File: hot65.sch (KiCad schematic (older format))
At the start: 158 parts, among them P1 USB_C_Plug_USB2.0, SW1 SW_Push, SW10 SW_Push, SW11 SW_Push, SW12 SW_Push, SW13 SW_Push, SW14 SW_Push, SW15 SW_Push, SW16 SW_Push, SW17 SW_Push, SW18 SW_Push, SW19 SW_Push, SW2 SW_Push, SW20 SW_Push, SW21 SW_Push, SW22 SW_Push, SW23 SW_Push, SW24 SW_Push, SW25 SW_Push, SW26 SW_Push, SW27 SW_Push, SW28 SW_Push, SW29 SW_Push, SW3 SW_Push, SW30 SW_Push, SW31 SW_Push, SW32 SW_Push, SW33 SW_Push, SW34 SW_Push, SW35 SW_Push, SW36 SW_Push, SW37 SW_Push, SW38 SW_Push, SW39 SW_Push, SW4 SW_Push, SW40 SW_Push, SW41 SW_Push, SW42 SW_Push, SW43 SW_Push, SW44 SW_Push, SW45 SW_Push, SW46 SW_Push, SW47 SW_Push, SW48 SW_Push, SW49 SW_Push, SW5 SW_Push, SW50 SW_Push, SW51 SW_Push, SW52 SW_Push, SW53 SW_Push, SW54 SW_Push, SW55 SW_Push, SW56 SW_Push, SW57 SW_Push, SW58 SW_Push, SW59 SW_Push, SW6 SW_Push, SW60 SW_Push, SW61 SW_Push, SW62 SW_Push, SW63 SW_Push, SW64 SW_Push, SW65 SW_Push, SW66 SW_Push, SW67 SW_Push, SW68 SW_Push, SW7 SW_Push, SW8 SW_Push, SW9 SW_Push, U1 ATmega32U4-AU, Y1 Crystal_Small

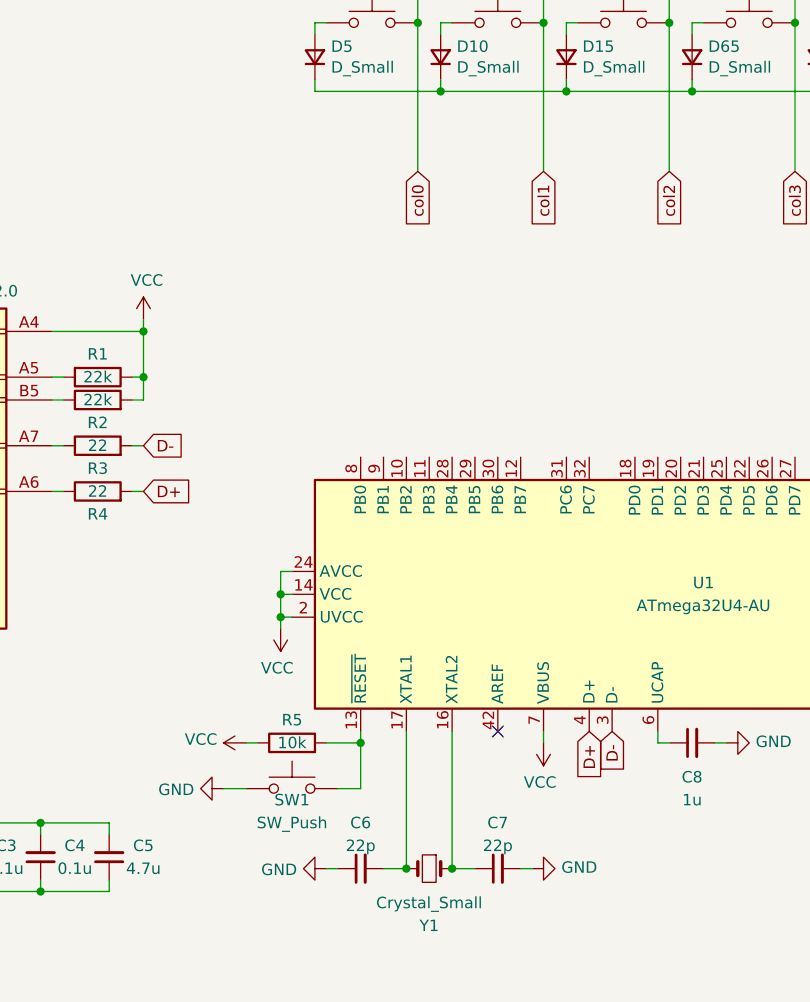
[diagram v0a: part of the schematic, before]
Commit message: v.0.7
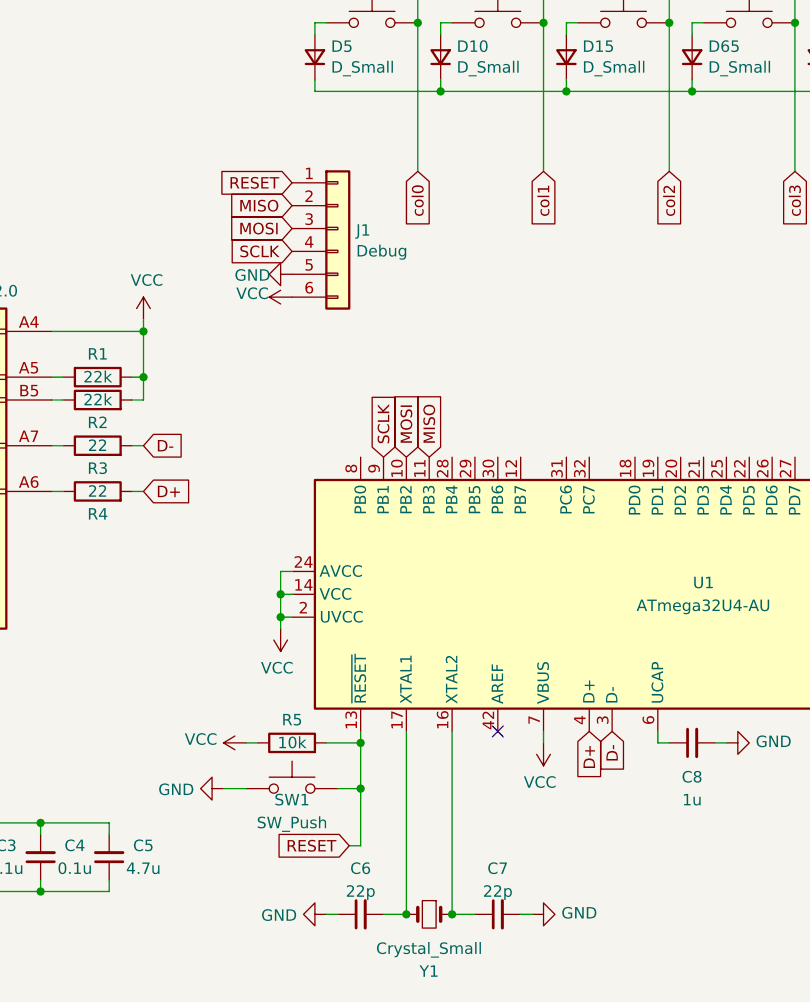
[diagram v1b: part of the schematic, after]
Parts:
- added J1: Debug, Connector_PinHeader_1.00mm:PinHeader_1x06_P1.00mm_Vertical, symbol Connector_Generic:Conn_01x06
- D1, D10, D11, D12, D13, D14, D15, D16, D17, D18, D19, D2, D20, D21, D22, D23, D24, D25, D26, D27, D28, D29, D3, D30, D31, D32, D33, D34, D35, D36, D37, D38, D39, D4, D40, D41, D42, D43, D44, D45, D46, D47, D48, D49, D5, D50, D51, D52, D53, D54, D55, D56, D57, D58, D59, D6, D60, D61, D62, D63, D64, D65, D66, D67, D7, D8, D9: footprint Diode_THT:D_A-405_P5.08mm_Vertical_AnodeUp -> Diode_THT:D_T-1_P5.08mm_Horizontal
- SW10, SW12, SW13, SW14, SW15, SW17, SW18, SW19, SW2, SW20, SW21, SW22, SW23, SW24, SW25, SW26, SW27, SW28, SW30, SW31, SW32, SW33, SW34, SW35, SW36, SW37, SW38, SW39, SW40, SW41, SW42, SW43, SW44, SW45, SW46, SW47, SW48, SW49, SW50, SW51, SW52, SW53, SW54, SW55, SW56, SW57, SW58, SW59, SW60, SW64, SW65, SW7, SW8, SW9: footprint keyswitches:Socket MX Alps -> MXSocketAlps:MXSocketAlps
- SW11, SW16, SW6: footprint keyswitches:Socket MX Alps -> MXSocketAlps:MXSocketAlps_1.25u
- SW29: footprint keyboardstuff:MXSocketAlps_6.25u -> MXSocketAlps:MXSocketAlps_6.25u
- SW3, SW62: footprint keyswitches:Socket MX Alps -> MXSocketAlps:MXSocketAlps_1.5u
- SW4: footprint keyswitches:Socket MX Alps -> MXSocketAlps:MXSocketAlps _1.75u
- SW5, SW61, SW66: footprint keyboardstuff:MXSocketAlps_2u -> MXSocketAlps:MXSocketAlps_2u
- SW63: footprint keyboardstuff:MXSocketAlps_2.25u -> MXSocketAlps:MXSocketAlps_2.25u
- SW67: footprint keyboardstuff:MXSocketAlps -> MXSocketAlps:MXSocketAlps_1.25u
- SW68: footprint keyboardstuff:MXSocketAlps_6.25u -> MXSocketAlps:MXSocketAlps_3u
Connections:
- net GND: now also J1.5 (Pin_5)
- net VCC: now also J1.6 (Pin_6)
- net MOSI: now reaches U1.10 (PB2)
- net MOSI: now also J1.3 (Pin_3)
- net MISO: now reaches U1.11 (PB3)
- net MISO: now also J1.2 (Pin_2)
- net RESET: now reaches R5.2, SW1.2, U1.13 (~RESET)
- net RESET: now also J1.1 (Pin_1)
- net SCLK: now reaches U1.9 (PB1)
- net SCLK: now also J1.4 (Pin_4)
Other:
- moved on the sheet: C6, C7, Y1

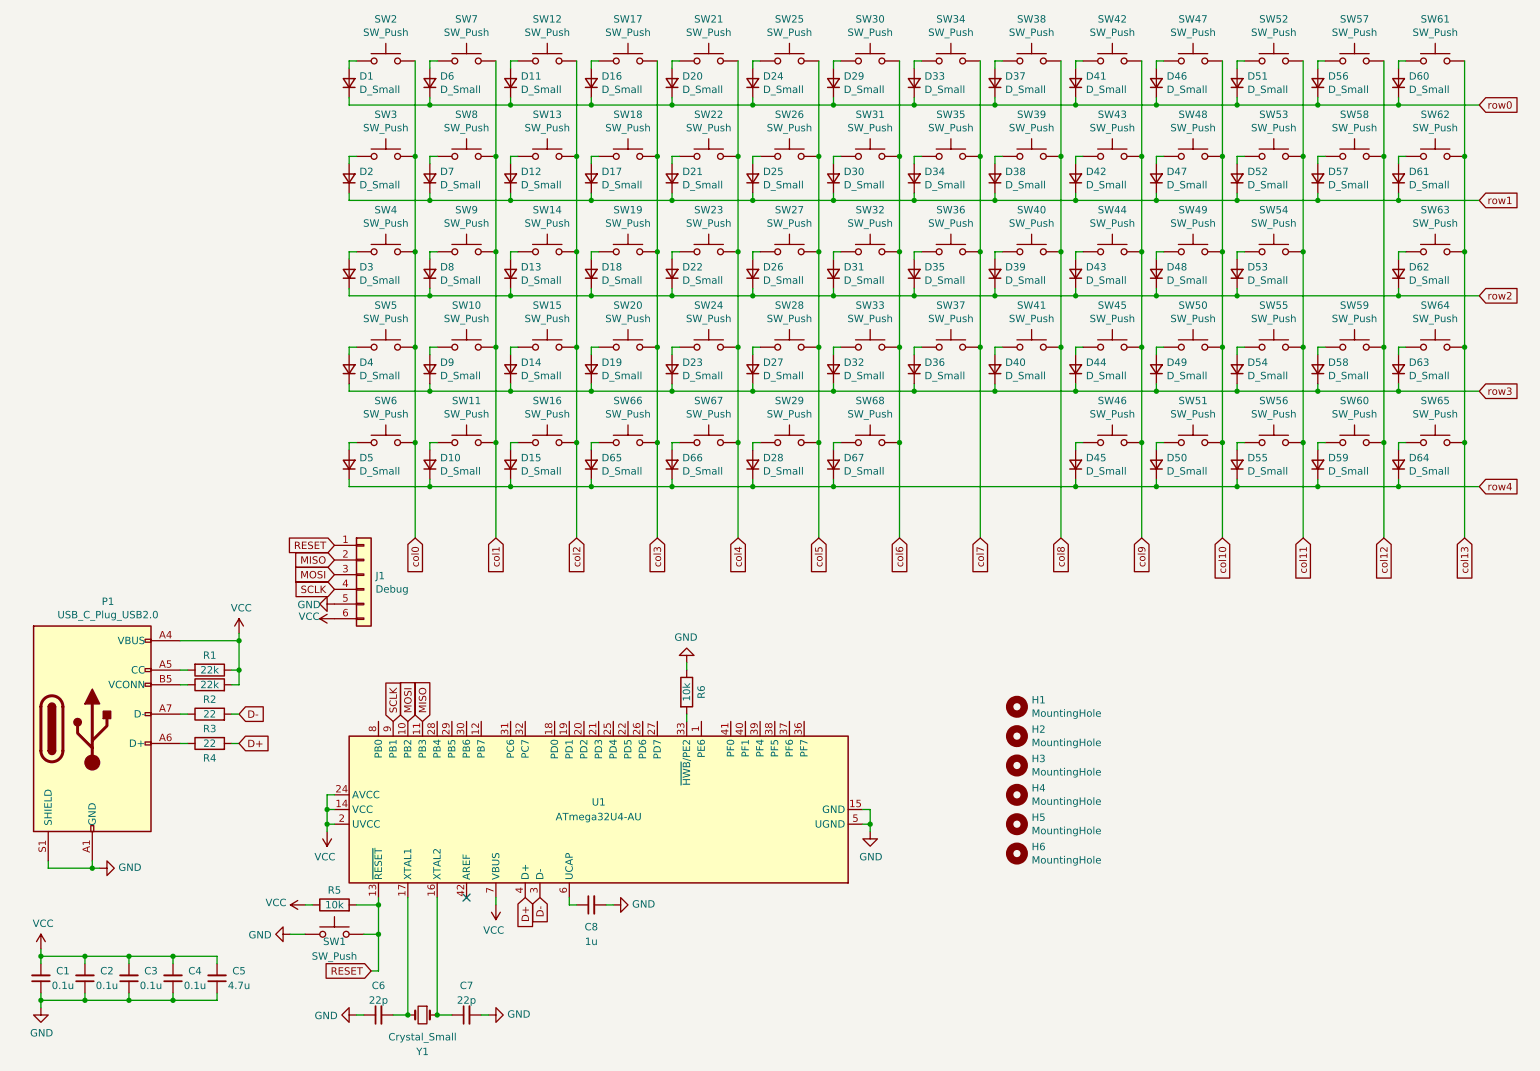
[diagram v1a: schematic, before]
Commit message: v.1.0
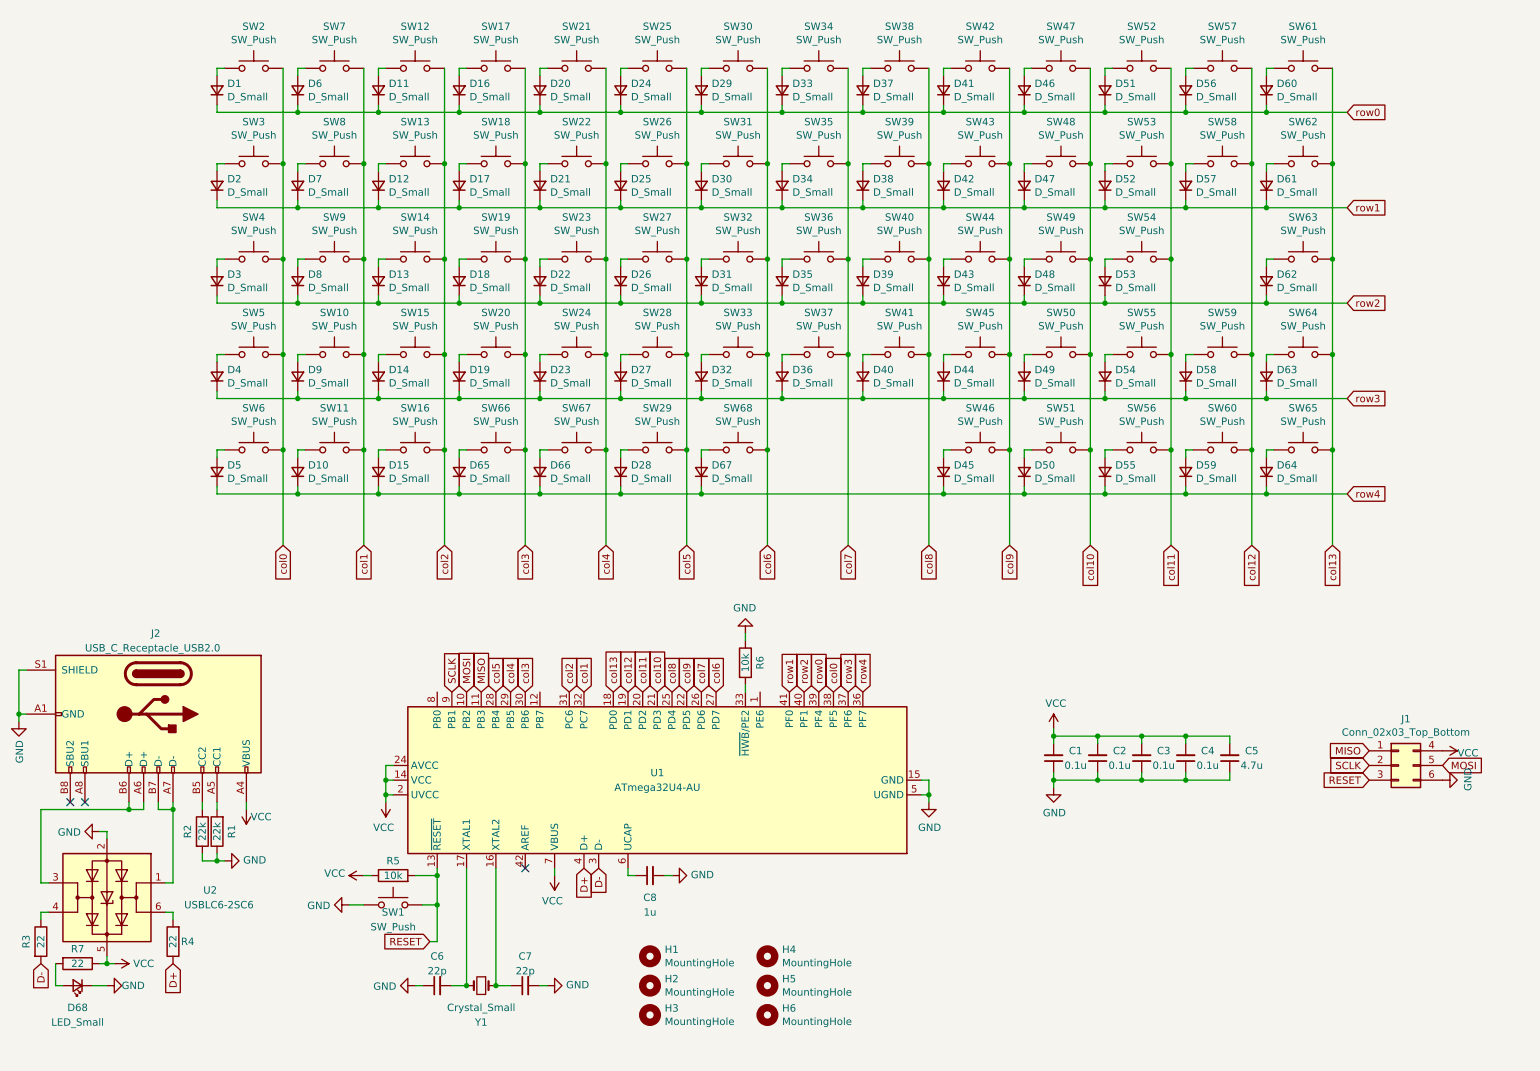
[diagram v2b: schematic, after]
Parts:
- removed J1: Debug, Connector_PinHeader_1.00mm:PinHeader_1x06_P1.00mm_Vertical, symbol Connector_Generic:Conn_01x06
- removed P1: USB_C_Plug_USB2.0, Connector_USB:USB_C_Receptacle_HRO_TYPE-C-31-M-12, symbol Connector:USB_C_Plug_USB2.0
- added D68: LED_Small, LED_SMD:LED_0603_1608Metric, symbol Device:LED_Small
- added J1: Conn_02x03_Top_Bottom, Connector_PinHeader_1.00mm:PinHeader_2x03_P1.00mm_Vertical, symbol Connector_Generic:Conn_02x03_Top_Bottom
- added J2: USB_C_Receptacle_USB2.0, Connector_USB:USB_C_Receptacle_XKB_U262-16XN-4BVC11, symbol Connector:USB_C_Receptacle_USB2.0
- added R7: 22, Resistor_SMD:R_0603_1608Metric_Pad0.98x0.95mm_HandSolder, symbol Device:R
- added U2: USBLC6-2SC6, Package_TO_SOT_SMD:SOT-23-6, symbol Power_Protection:USBLC6-2SC6
- H1, H2, H3, H4: footprint MountingHole:MountingHole_2.2mm_M2_DIN965 -> keyboardstuff:M2_slot
- H5, H6: footprint MountingHole:MountingHole_2.2mm_M2_DIN965 -> keyboardstuff:M2_long_slot
- SW4: footprint MXSocketAlps:MXSocketAlps _1.75u -> MXSocketAlps:MXSocketAlps_1.75u
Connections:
- net D+: now also R4.1; no longer R4.2
- net GND: now also R1.1, R2.2, D68.1 (K), J1.6 (Pin_6), J2.A1 (GND), J2.A12 (GND), J2.B1 (GND), J2.B12 (GND), J2.S1 (SHIELD), U2.2 (GND)
- net MISO: now also J1.1 (Pin_1)
- net MOSI: now also J1.5 (Pin_5)
- net RESET: now also J1.3 (Pin_3)
- net SCLK: now also J1.2 (Pin_2)
- net VCC: now also J1.4 (Pin_4), J2.A4 (VBUS), J2.A9 (VBUS), J2.B4 (VBUS), J2.B9 (VBUS), R7.1, U2.5 (VBUS); no longer R1.1, R2.2
- net col0: now also U1.38 (PF5)
- net col1: now also U1.32 (PC7)
- net col10: now also U1.21 (PD3)
- net col11: now also U1.20 (PD2)
- net col12: now also U1.19 (PD1)
- net col13: now also U1.18 (PD0)
- net col2: now also U1.31 (PC6)
- net col3: now also U1.30 (PB6)
- net col4: now also U1.29 (PB5)
- net col5: now also U1.28 (PB4)
- net col6: now also U1.27 (PD7)
- net col7: now also U1.26 (PD6)
- net col8: now also U1.25 (PD4)
- net col9: now also U1.22 (PD5)
- net row0: now also U1.39 (PF4)
- net row1: now also U1.41 (PF0)
- net row2: now also U1.40 (PF1)
- net row3: now also U1.37 (PF6)
- net row4: now also U1.36 (PF7)
- net at R1.2: now also J2.A5 (CC1)
- net at R3.1: now also U2.4 (I/O2)
- net at R2.1: now also J2.B5 (CC2)
- new net: J2.A6 (D+), J2.B6 (D+), U2.3 (I/O2)
- new net: J2.A7 (D-), J2.B7 (D-), U2.1 (I/O1)
- new net: R4.2, U2.6 (I/O1)
- new net: D68.2 (A), R7.2
- no-connect marks 1 -> 3
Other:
- moved on the sheet: C1, C2, C3, C4, C5, C6, C7, C8, D1, D10, D11, D12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
